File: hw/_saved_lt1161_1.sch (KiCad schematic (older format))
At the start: 8 parts, among them U501 BTS6133D, U502 BTS6133D, U503 BTS6133D, U504 BTS6133D

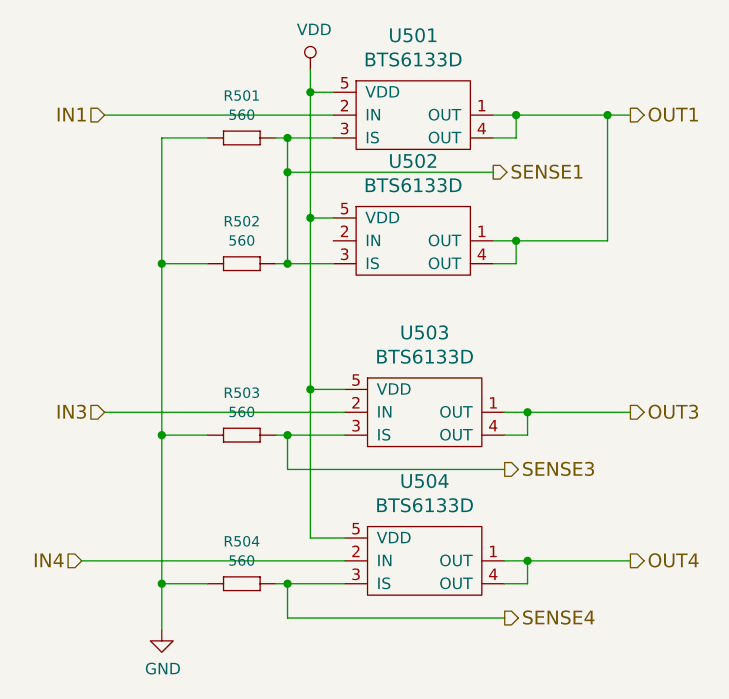
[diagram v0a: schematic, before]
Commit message: 3.0.0 ready to order
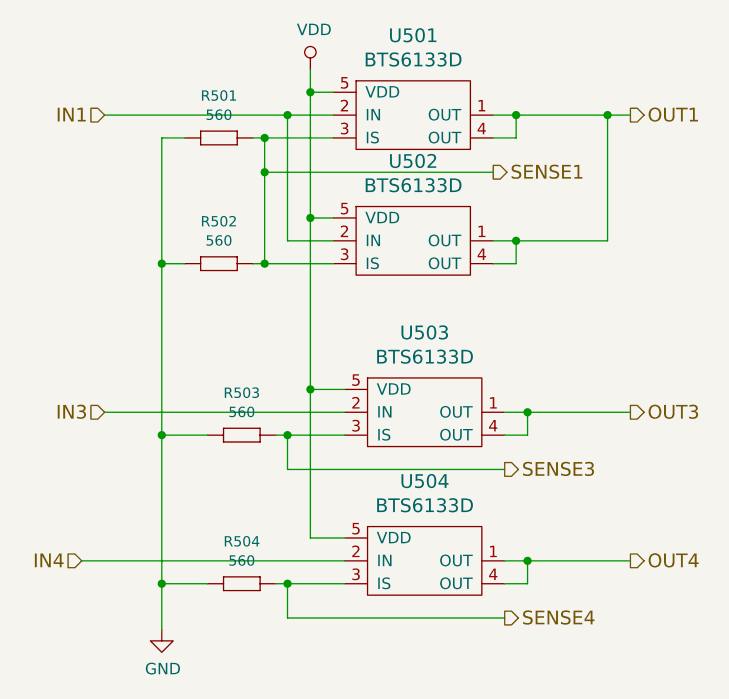
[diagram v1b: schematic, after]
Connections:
- net IN1: now also U502.2 (IN)
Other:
- moved on the sheet: R501, R502
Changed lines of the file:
@@
 L 560 R501
 U 1 1 59D7D931
-P 4250 3300
-F 0 "R501" H 4300 3484 45  0000 C CNN
-F 1 "560" H 4300 3400 45  0000 C CNN
-F 2 "yageo:0603" H 4280 3450 20  0001 C CNN
-F 3 "" H 4219 3339 60  0001 C CNN
-F 4 "" H 4619 3739 60  0001 C CNN "1st Source Part Number"
-F 5 "Digikey" H 4519 3639 60  0001 C CNN "1st Source"
-F 6 "RC0603FR-07560RL" H 4419 3539 60  0001 C CNN "Manufacturer Part Number"
-F 7 "YAGEO" H 4319 3439 60  0001 C CNN "Manufacturer"
-	1    4250 3300
+P 4150 3300
+F 0 "R501" H 4200 3484 45  0000 C CNN
+F 1 "560" H 4200 3400 45  0000 C CNN
+F 2 "yageo:0603" H 4180 3450 20  0001 C CNN
+F 3 "" H 4119 3339 60  0001 C CNN
+F 4 "" H 4519 3739 60  0001 C CNN "1st Source Part Number"
+F 5 "Digikey" H 4419 3639 60  0001 C CNN "1st Source"
+F 6 "RC0603FR-07560RL" H 4319 3539 60  0001 C CNN "Manufacturer Part Number"
+F 7 "YAGEO" H 4219 3439 60  0001 C CNN "Manufacturer"
+	1    4150 3300
 	1    0    0    -1
 $EndComp
 Wire Wire Line
-	4450 3300 4700 3300
+	4350 3300 4700 3300
 $Comp
 L 560 R502
 U 1 1 59D7DE83
-P 4250 3850
-F 0 "R502" H 4300 4034 45  0000 C CNN
-F 1 "560" H 4300 3950 45  0000 C CNN
-F 2 "yageo:0603" H 4280 4000 20  0001 C CNN
-F 3 "" H 4219 3889 60  0001 C CNN
-F 4 "" H 4619 4289 60  0001 C CNN "1st Source Part Number"
-F 5 "Digikey" H 4519 4189 60  0001 C CNN "1st Source"
-F 6 "RC0603FR-07560RL" H 4419 4089 60  0001 C CNN "Manufacturer Part Number"
-F 7 "YAGEO" H 4319 3989 60  0001 C CNN "Manufacturer"
-	1    4250 3850
+P 4150 3850
+F 0 "R502" H 4200 4034 45  0000 C CNN
+F 1 "560" H 4200 3950 45  0000 C CNN
+F 2 "yageo:0603" H 4180 4000 20  0001 C CNN
+F 3 "" H 4119 3889 60  0001 C CNN
+F 4 "" H 4519 4289 60  0001 C CNN "1st Source Part Number"
+F 5 "Digikey" H 4419 4189 60  0001 C CNN "1st Source"
+F 6 "RC0603FR-07560RL" H 4319 4089 60  0001 C CNN "Manufacturer Part Number"
+F 7 "YAGEO" H 4219 3989 60  0001 C CNN "Manufacturer"
+	1    4150 3850
 	1    0    0    -1
 $EndComp
 Wire Wire Line
-	4450 3850 4700 3850
+	4350 3850 4700 3850
 Wire Wire Line
-	4500 3300 4500 3850
-Connection ~ 4500 3300
-Connection ~ 4500 3850
+	4400 3300 4400 3850
+Connection ~ 4400 3300
+Connection ~ 4400 3850
 $Comp
 L GND #PWR023
@@
 	3950 3300 3950 5450
 Wire Wire Line
-	3950 3300 4150 3300
+	3950 3300 4050 3300
 Wire Wire Line
-	4150 3850 3950 3850
+	4050 3850 3950 3850
 Connection ~ 3950 3850
 $Comp
@@
 	3600 5150 4750 5150
 Wire Wire Line
-	5400 3450 4500 3450
-Connection ~ 4500 3450
+	5400 3450 4400 3450
+Connection ~ 4400 3450
 Wire Wire Line
 	5450 4750 4500 4750
@@
 	5900 3750 5900 3200
 Connection ~ 5900 3200
+Wire Wire Line
+	4700 3750 4500 3750
+Wire Wire Line
+	4500 3750 4500 3200
+Connection ~ 4500 3200
 $EndSCHEMATC
